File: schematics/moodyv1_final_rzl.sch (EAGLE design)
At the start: 9 parts, among them Q1 IRLML5203

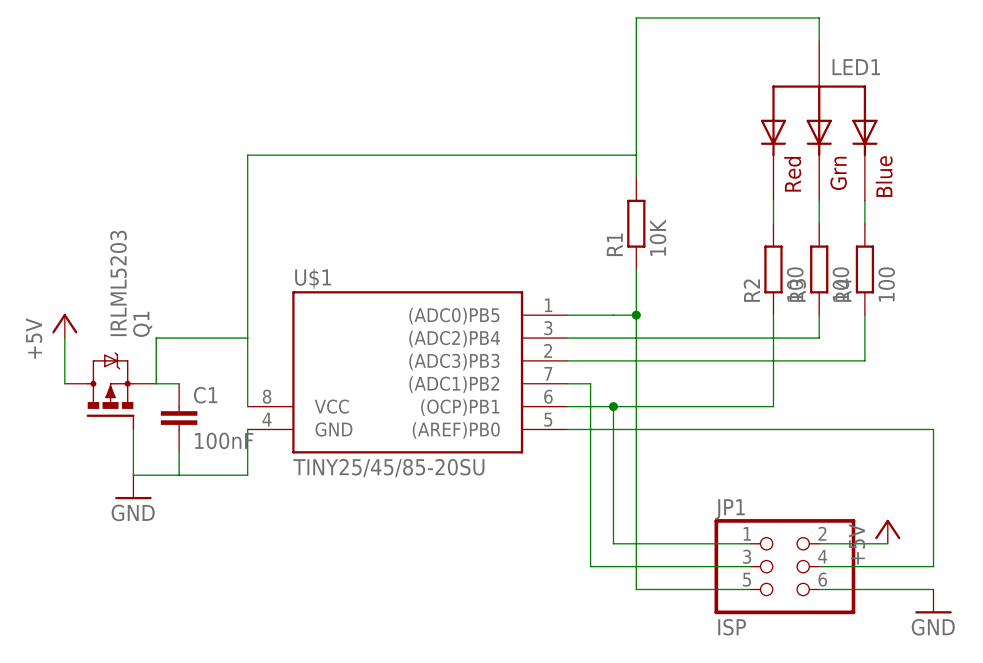
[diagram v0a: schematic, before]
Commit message: add newest schematic
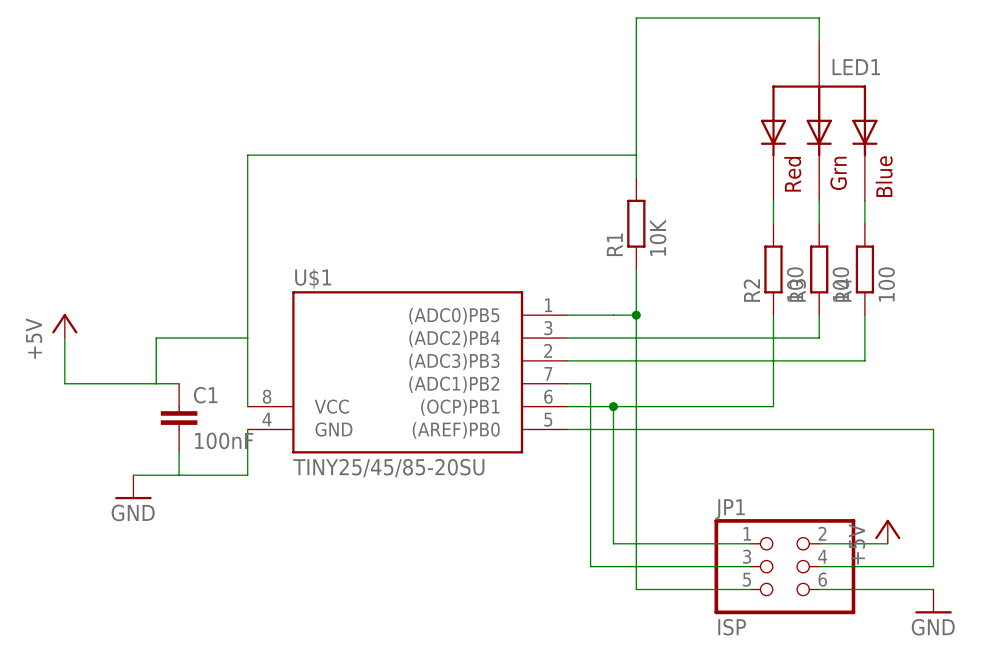
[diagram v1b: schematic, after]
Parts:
- removed Q1: IRLML5203, transistor-power:IRLML5203
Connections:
- removed net N$1: C1.1, LED1.VCC, Q1.S, R1.2, U$1.VCC
- net +5V: now also C1.1, LED1.VCC, R1.2, U$1.VCC; no longer Q1.D
- net GND: no longer Q1.G
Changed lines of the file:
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@@
 <part name="P+3" library="supply1" deviceset="+5V" device=""/>
 <part name="GND2" library="supply1" deviceset="GND" device=""/>
-<part name="Q1" library="transistor-power" deviceset="IRLML5203" device=""/>
 <part name="C1" library="resistor" deviceset="C-EU" device="C0805" value="100nF"/>
 </parts>
@@
 <instance part="P+3" gate="1" x="116.84" y="30.48"/>
 <instance part="GND2" gate="1" x="121.92" y="20.32"/>
-<instance part="Q1" gate="G$1" x="30.48" y="43.18" rot="MR90"/>
 <instance part="C1" gate="G$1" x="38.1" y="43.18"/>
 </instances>
@@
 <pinref part="U$1" gate="G$1" pin="GND"/>
 <wire x1="45.72" y1="40.64" x2="45.72" y2="35.56" width="0.1524" layer="91"/>
-<pinref part="Q1" gate="G$1" pin="G"/>
 <wire x1="45.72" y1="35.56" x2="38.1" y2="35.56" width="0.1524" layer="91"/>
 <wire x1="38.1" y1="35.56" x2="33.02" y2="35.56" width="0.1524" layer="91"/>
-<wire x1="33.02" y1="40.64" x2="33.02" y2="35.56" width="0.1524" layer="91"/>
 <pinref part="C1" gate="G$1" pin="2"/>
 <wire x1="38.1" y1="38.1" x2="38.1" y2="35.56" width="0.1524" layer="91"/>
@@
 <segment>
 <pinref part="P+1" gate="1" pin="+5V"/>
-<pinref part="Q1" gate="G$1" pin="D"/>
 <wire x1="25.4" y1="50.8" x2="25.4" y2="45.72" width="0.1524" layer="91"/>
-</segment>
-</net>
-<net name="N$1" class="0">
-<segment>
-<pinref part="Q1" gate="G$1" pin="S"/>
 <pinref part="U$1" gate="G$1" pin="VCC"/>
 <wire x1="35.56" y1="45.72" x2="35.56" y2="50.8" width="0.1524" layer="91"/>
@@
 <pinref part="C1" gate="G$1" pin="1"/>
 <wire x1="35.56" y1="45.72" x2="38.1" y2="45.72" width="0.1524" layer="91"/>
+<wire x1="25.4" y1="45.72" x2="35.56" y2="45.72" width="0.1524" layer="91"/>
 </segment>
 </net>
